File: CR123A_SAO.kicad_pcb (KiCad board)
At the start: 2 copper layers, 15 parts, among them J1 Conn_02x03_Odd_Even, P1 USB_C_Plug_USB2.0, SW1 SW_SPDT_1825232-1, U2 MT2492

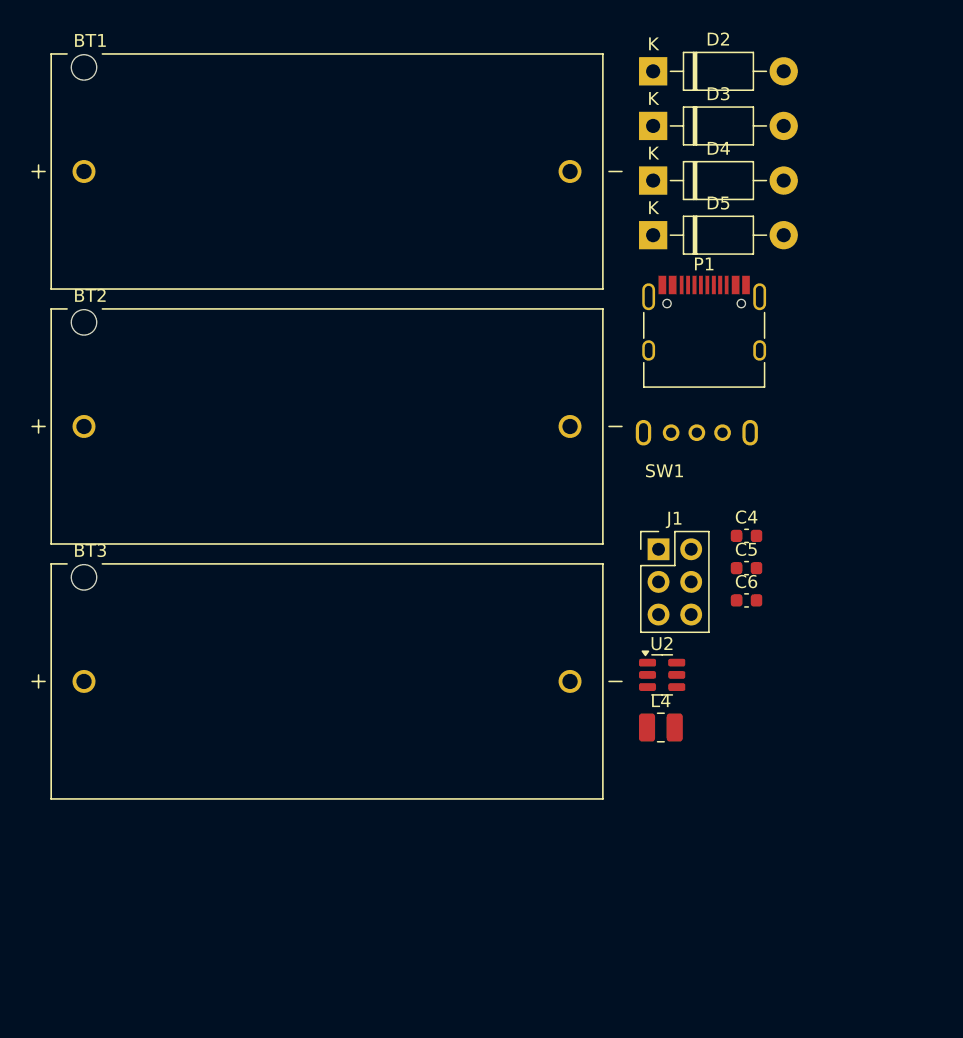
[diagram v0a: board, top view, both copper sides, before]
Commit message: sent to jlcpcb
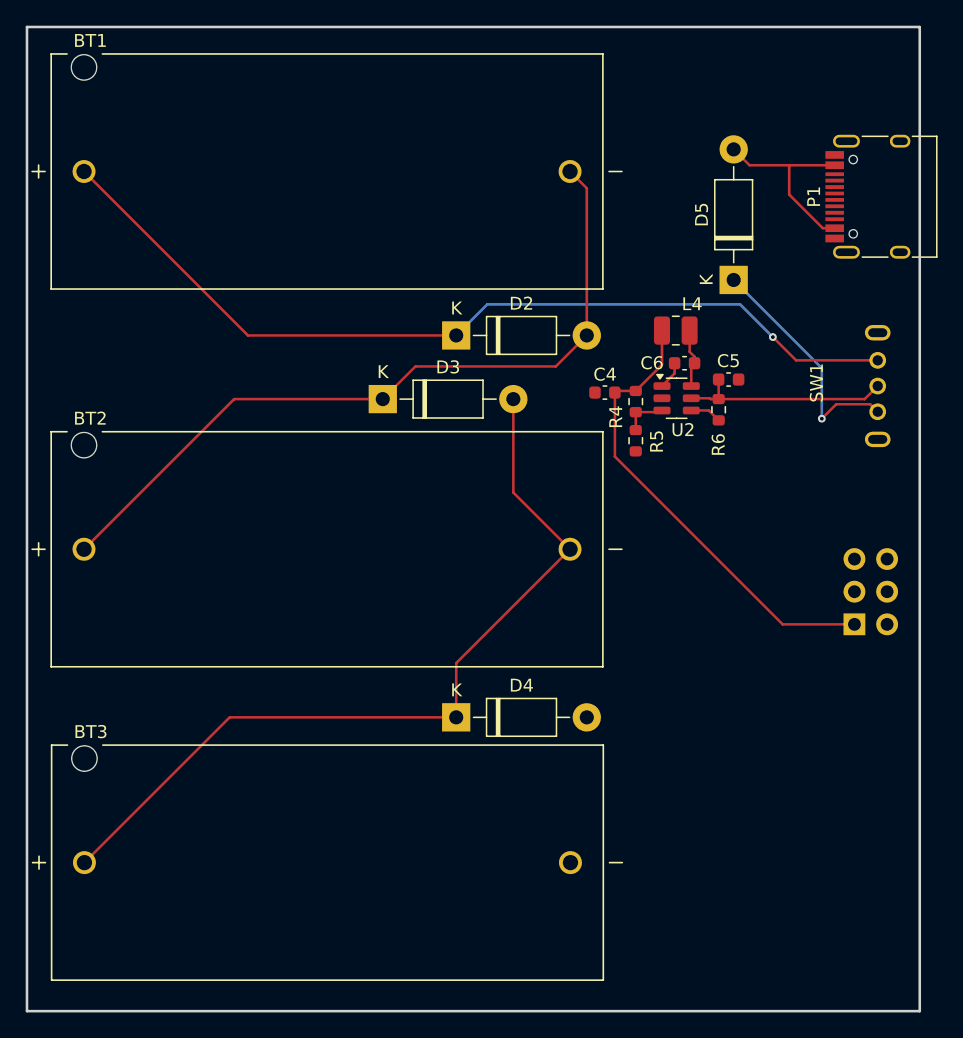
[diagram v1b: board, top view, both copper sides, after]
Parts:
- added R4: 36k, Resistor_SMD:R_0603_1608Metric, F.Cu at (57.9, 43.1)
- added R5: 8k, Resistor_SMD:R_0603_1608Metric, F.Cu at (57.9, 46.2)
- added R6: 8k, Resistor_SMD:R_0603_1608Metric, F.Cu at (64.4, 43.8)
- J1: moved to B.Cu
- moved D4 44.5 mm to (43.9, 67.7)
- moved L4 30.9 mm to (61.0, 37.6)
- moved D3 29.9 mm to (38.2, 42.9)
- moved D2 25.6 mm to (43.9, 38.0)
- moved U2 21.6 mm to (61.1, 42.9)
- moved C6 19.1 mm to (61.7, 40.1), turned to 180 degrees
- moved P1 17.9 mm to (77.4, 27.2), turned to 90 degrees
- moved J1 16.3 mm to (74.9, 60.5)
- moved C4 15.7 mm to (55.5, 42.4), turned to 180 degrees
- moved C5 14.7 mm to (65.1, 41.4)
- moved SW1 14.5 mm to (76.7, 41.9), turned to 90 degrees
- moved BT3 14.1 mm to (33.9, 79.0)
- moved BT2 9.55 mm to (33.9, 54.6)
- moved D5 7.17 mm to (65.5, 33.7), turned to 90 degrees
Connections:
- SW1 pad 3: unconnected-(SW1-C-Pad3) -> +9V
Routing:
- net +9V: track 0.00 -> 69.8 mm, vias 0 -> 1
- net Net-(D3-A): track 0.00 -> 63.9 mm
- net Net-(D2-A): track 0.00 -> 59.3 mm
- net VCC: track 0.00 -> 36.3 mm
- net +5V: track 0.00 -> 18.7 mm, vias 0 -> 1
- net VDC: track 0.00 -> 16.5 mm
- net Net-(D5-A): track 0.00 -> 15.3 mm
- net Net-(U2-SW): track 0.00 -> 4.58 mm
- net Net-(U2-FB): track 0.00 -> 3.50 mm
- net Net-(U2-EN): track 0.00 -> 2.45 mm
- net Net-(U2-BS): track 0.00 -> 2.18 mm
- added copper zone on F.Cu, net GND
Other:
- board outline added: 69.5 x 76.6 mm
